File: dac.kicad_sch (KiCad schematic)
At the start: 9 parts

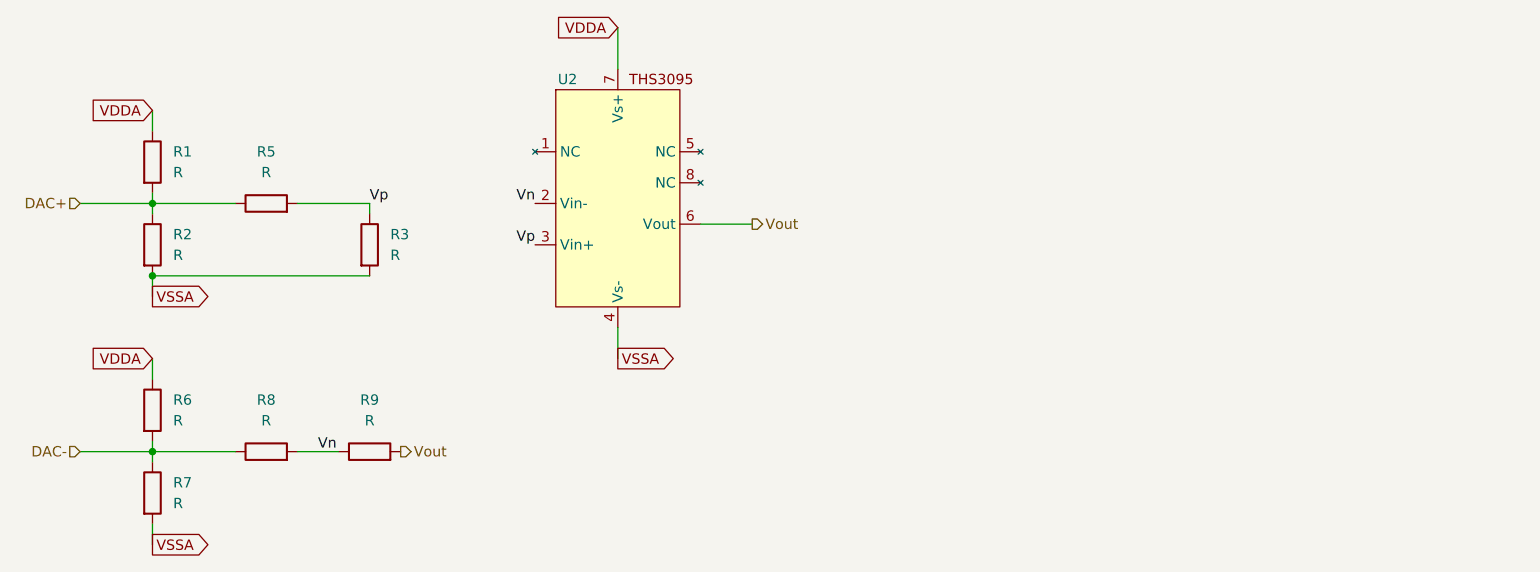
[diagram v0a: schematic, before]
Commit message: feat: added Larry's goofy ahh + finished my schematic
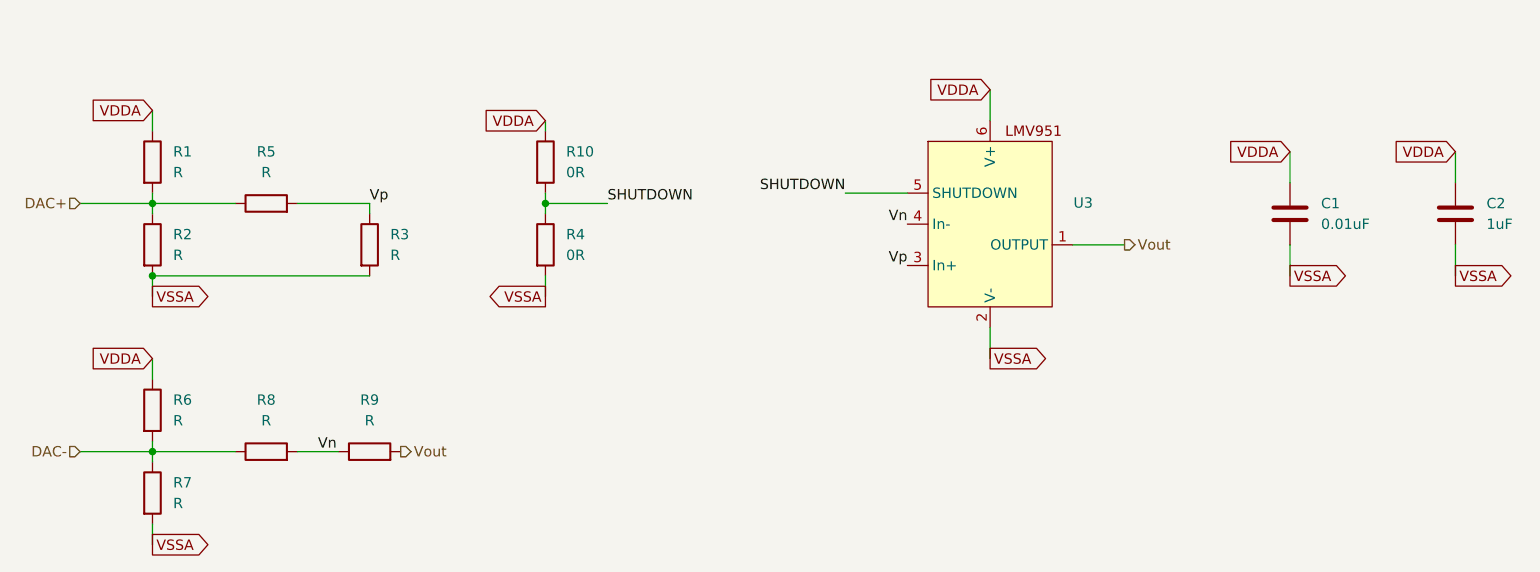
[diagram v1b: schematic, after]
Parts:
- removed U2: ~, symbol dac:THS3095
- added C1: 0.01uF, symbol Device:C
- added C2: 1uF, symbol Device:C
- added R10, R4: 0R, Resistor_SMD:R_0201_0603Metric, symbol Device:R
- added U3: ~, Package_TO_SOT_SMD:TSOT-23-6, symbol dac:LMV951
- R1, R2, R3, R5, R6, R7, R8, R9: footprint (none) -> Resistor_SMD:R_0201_0603Metric
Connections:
- net VDDA: now also C1.1, C2.1, R10.1, U3.6 (V+)
- net VSSA: now also C1.2, C2.2, R4.2, U3.2 (V-)
- net Vn: now also U3.4 (In-)
- net Vout: now also U3.1 (OUTPUT)
- net Vp: now also U3.3 (In+)
- new net SHUTDOWN: R10.2, R4.1, U3.5 (SHUTDOWN)
